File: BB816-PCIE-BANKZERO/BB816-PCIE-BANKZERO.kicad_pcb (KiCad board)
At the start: 4 copper layers, 167.6 x 111.2 mm, 20 parts, among them J1 BB816_BreakoutA27_PCIex16, J1 Bypass, U1 AS7C256B-15PIN, U10 74HC138, U15 74HC32, U16 74HC138, U18 74HC00, U2 AS7C256B-15PIN, U23 74HC04, U3 AT28C256-15PU, U4 74HC138, U5 74HC148, U6 74HC125, U7 74HC283, U9 74HC32

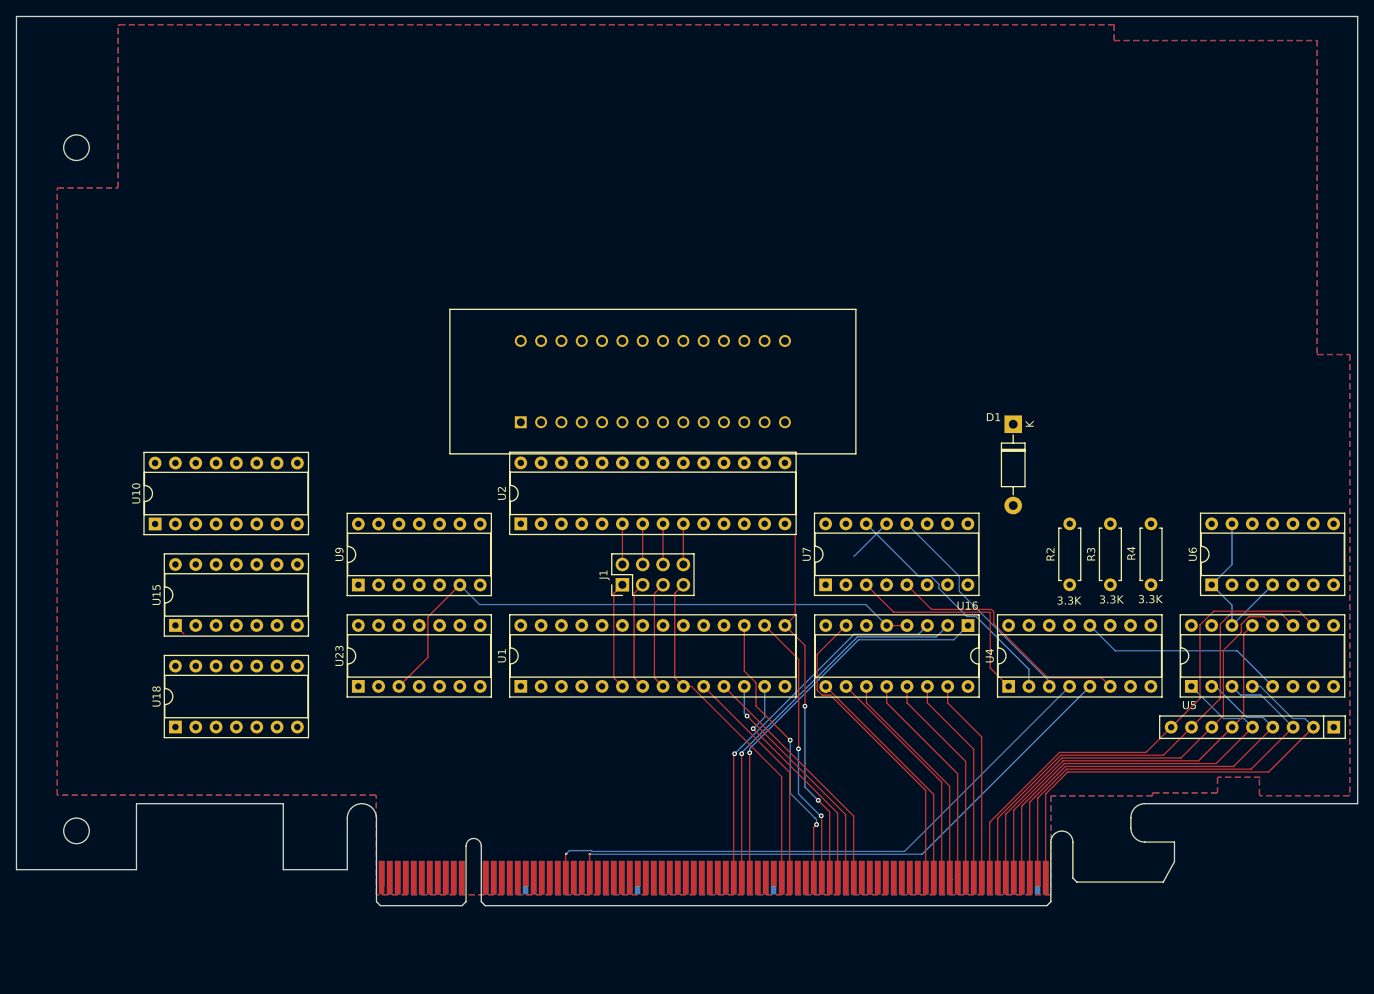
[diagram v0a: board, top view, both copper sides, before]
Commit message: Bum AND
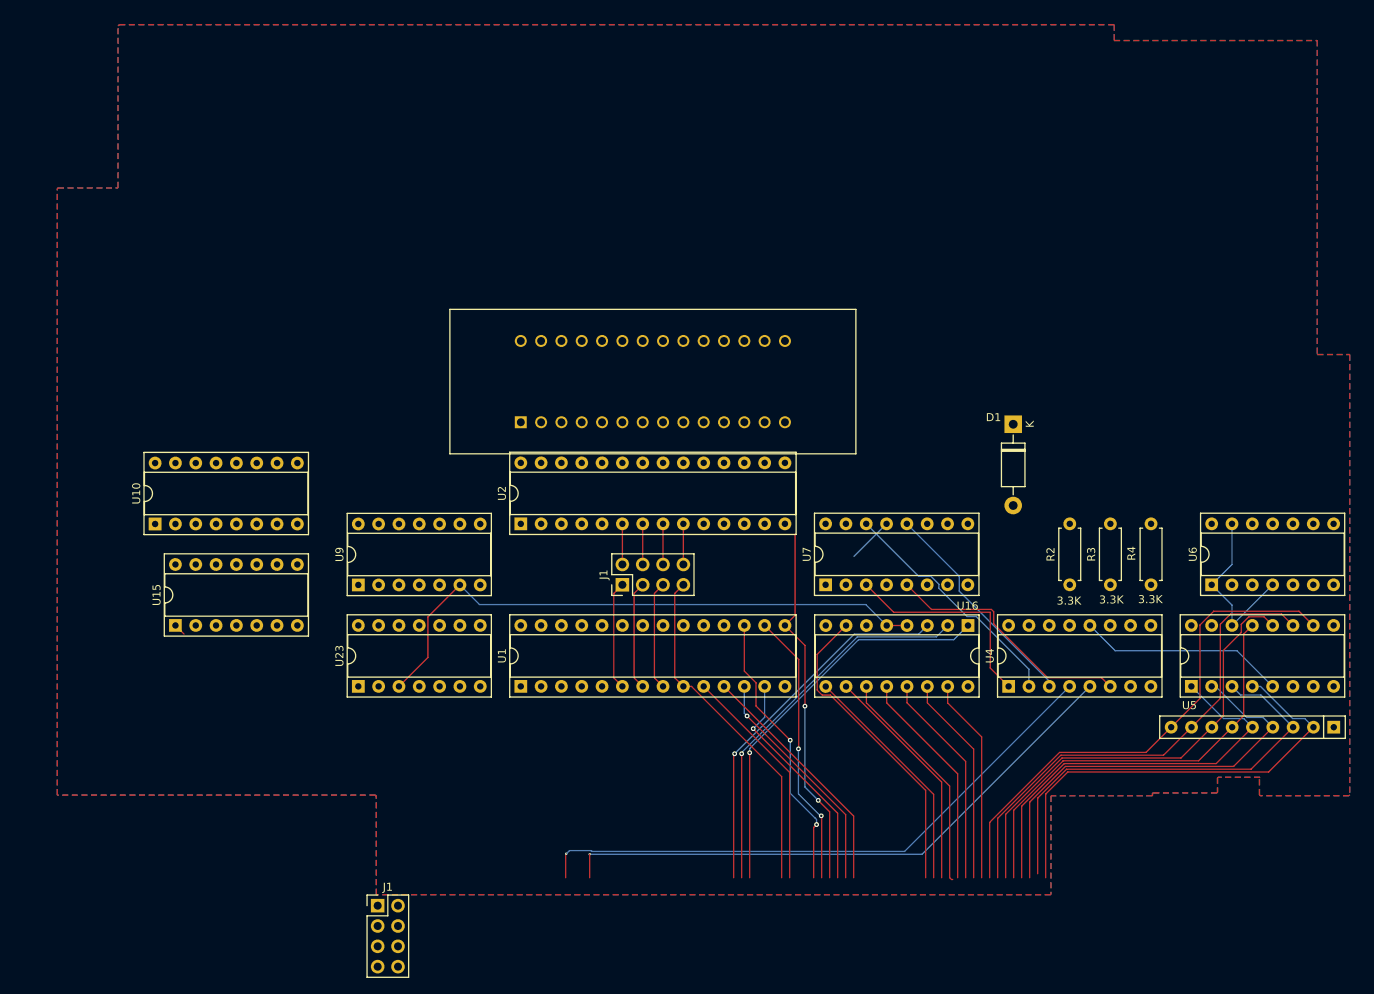
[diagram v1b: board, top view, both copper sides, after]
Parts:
- removed U18: 74HC00, Package_DIP:DIP-14_W7.62mm_Socket
- J1: value BB816_BreakoutA27_PCIex16 -> Bypass; footprint BB816-MATX-PCIE:PCIexpress_x16_HW_FH -> Connector_PinHeader_2.54mm:PinHeader_2x04_P2.54mm_Vertical
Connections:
- U23 pad 1: /~{RAM0_OE} -> (no net)
- U23 pad 2: /RD -> (no net)
- U6 pad 10: VCC -> /~{RAM0_OE}
- U6 pad 8: unconnected-(U6-Pad8) -> /EMU_RD
- U6 pad 9: GND -> /E
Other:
- board outline removed
